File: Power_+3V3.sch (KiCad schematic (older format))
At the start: 10 parts

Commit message: Add files via upload
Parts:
- removed C? (x2): 10u, Capacitor_SMD:C_1206_3216Metric_Pad1.33x1.80mm_HandSolder, symbol Device:C
- removed C?: 0,1, Capacitor_SMD:C_0603_1608Metric_Pad1.08x0.95mm_HandSolder, symbol Device:C
- removed C?: 1u, Capacitor_SMD:C_0603_1608Metric_Pad1.08x0.95mm_HandSolder, symbol Device:C
- removed D?: SMAJ5.0CA, symbol Device:D_TVS
- removed TP?: TestPoint, symbol Connector:TestPoint
- removed U?: AMS1117-3.3, Package_TO_SOT_SMD:SOT-223-3_TabPin2, symbol Regulator_Linear:AMS1117-3.3
- added C? (x2): 10u, Capacitor_SMD:C_1206_3216Metric_Pad1.33x1.80mm_HandSolder, symbol Device:C
- added C?: 0,1, Capacitor_SMD:C_0603_1608Metric_Pad1.08x0.95mm_HandSolder, symbol Device:C
- added C?: 1u, Capacitor_SMD:C_0603_1608Metric_Pad1.08x0.95mm_HandSolder, symbol Device:C
- added TP?: TestPoint, symbol Connector:TestPoint
- added U?: AMS1117-3.3, Package_TO_SOT_SMD:SOT-223-3_TabPin2, symbol Regulator_Linear:AMS1117-3.3
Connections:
- wire segments 18 -> 16

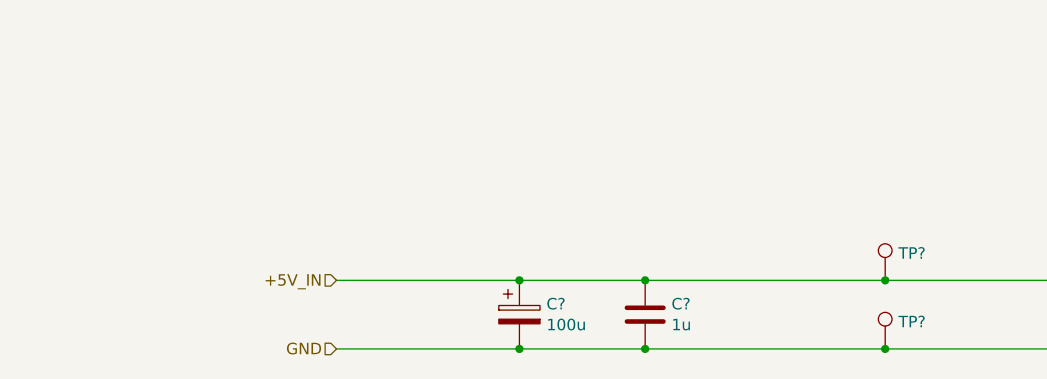
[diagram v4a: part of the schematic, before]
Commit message: Add files via upload
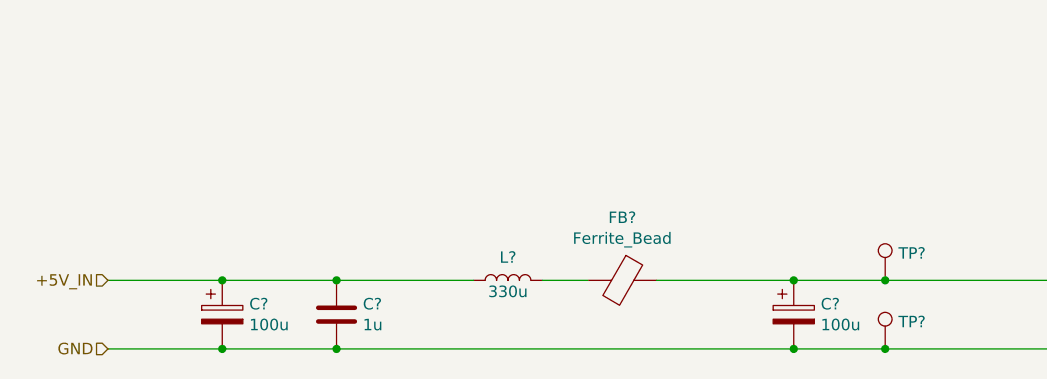
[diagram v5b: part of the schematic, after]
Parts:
- removed C?: 100u, symbol Device:CP
- removed C?: 1u, Capacitor_SMD:C_0603_1608Metric_Pad1.08x0.95mm_HandSolder, symbol Device:C
- added C?: 1u, Capacitor_SMD:C_0603_1608Metric_Pad1.08x0.95mm_HandSolder, symbol Device:C
- added C? (x2): 100u, symbol Device:CP
- added FB?: Ferrite_Bead, symbol Device:Ferrite_Bead
- added L?: 330u, symbol Device:L
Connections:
- net +5V_IN: now also C?.1, C?.1, L?.1; no longer C?.1, TP?.1, U?.3 (VI)
- net GND: now also C?.2, C?.2, C?.2
- new net: C?.1, C?.1, FB?.1, TP?.1, U?.3 (VI)
- new net: FB?.2, L?.2
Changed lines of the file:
@@
 $Descr A4 11693 8268
 encoding utf-8
-Sheet 13 23
+Sheet 11 23
 Title ""
 Date ""
@@
 	1    0    0    -1
 $EndComp
-$Comp
-L Device:C C?
-U 1 1 60E73028
-P 4350 3650
-AR Path="/60E73028" Ref="C?"  Part="1"
-AR Path="/609CA6A8/609D24C0/60E73028" Ref="C?"  Part="1"
-AR Path="/609CA6A8/60A08E0B/60E73028" Ref="C?"  Part="1"
-AR Path="/609CA6A8/60A0A46E/60E73028" Ref="C?"  Part="1"
-AR Path="/609CA6A8/60A0A500/60E73028" Ref="C?"  Part="1"
-AR Path="/609CA6A8/60A0A922/60E73028" Ref="C?"  Part="1"
-AR Path="/609CA6A8/60E73028" Ref="C?"  Part="1"
-AR Path="/609CA6A8/60AE5653/60E73028" Ref="C?"  Part="1"
-AR Path="/609FED99/60E73028" Ref="C?"  Part="1"
-AR Path="/60DF07DE/60E73028" Ref="C?"  Part="1"
-AR Path="/60DF0860/60E73028" Ref="C?"  Part="1"
-AR Path="/60DF1072/60E73028" Ref="C?"  Part="1"
-AR Path="/60DF1160/60E73028" Ref="C?"  Part="1"
-AR Path="/60DF196E/60E73028" Ref="C?"  Part="1"
-AR Path="/60DF212D/60E73028" Ref="C?"  Part="1"
-AR Path="/60E6F2E9/60E73028" Ref="C?"  Part="1"
-F 0 "C?" H 4465 3696 50  0000 L CNN
-F 1 "1u" H 4465 3605 50  0000 L CNN
-F 2 "Capacitor_SMD:C_0603_1608Metric_Pad1.08x0.95mm_HandSolder" H 4388 3500 50  0001 C CNN
-F 3 "~" H 4350 3650 50  0001 C CNN
-	1    4350 3650
-	1    0    0    -1
-$EndComp
-$Comp
-L Device:CP C?
-U 1 1 60DF19BC
-P 3800 3650
-AR Path="/609FED99/60DF19BC" Ref="C?"  Part="1"
-AR Path="/60DF07DE/60DF19BC" Ref="C?"  Part="1"
-AR Path="/60DF0860/60DF19BC" Ref="C?"  Part="1"
-AR Path="/60DF1072/60DF19BC" Ref="C?"  Part="1"
-AR Path="/60DF1160/60DF19BC" Ref="C?"  Part="1"
-AR Path="/60DF196E/60DF19BC" Ref="C?"  Part="1"
-AR Path="/60DF212D/60DF19BC" Ref="C?"  Part="1"
-AR Path="/60E6F2E9/60DF19BC" Ref="C?"  Part="1"
-F 0 "C?" H 3918 3696 50  0000 L CNN
-F 1 "100u" H 3918 3605 50  0000 L CNN
-F 2 "" H 3838 3500 50  0001 C CNN
-F 3 "~" H 3800 3650 50  0001 C CNN
-	1    3800 3650
-	1    0    0    -1
-$EndComp
-Text HLabel 3000 3500 0    50   Input ~ 0
+Text HLabel 2000 3500 0    50   Input ~ 0
 +5V_IN
-Wire Wire Line
-	3000 3500 3800 3500
 Connection ~ 6200 3500
-Connection ~ 3800 3500
-Wire Wire Line
-	3800 3500 4350 3500
-Connection ~ 4350 3500
-Connection ~ 5400 3500
-Wire Wire Line
-	3800 3800 4350 3800
 Connection ~ 6200 3800
-Connection ~ 4350 3800
 Wire Wire Line
 	6800 3800 7400 3800
-Wire Wire Line
-	3000 3800 3800 3800
-Connection ~ 3800 3800
 $Comp
 L Connector:TestPoint TP?
@@
 	1    0    0    -1
 $EndComp
-Connection ~ 5400 3800
 Wire Wire Line
 	7400 3500 7550 3500
@@
 	7550 3500 7800 3500
 Connection ~ 7550 3500
-Text HLabel 3000 3800 0    50   Input ~ 0
+Text HLabel 2000 3800 0    50   Input ~ 0
 GND
 Text Notes 6900 2250 2    197  ~ 0
@@
 	7800 3500 8500 3500
 Connection ~ 7800 3500
-Wire Wire Line
-	4350 3800 5400 3800
-Wire Wire Line
-	4350 3500 5400 3500
+$Comp
+L Device:C C?
+U 1 1 60FB3F89
+P 3000 3650
+AR Path="/60FB3F89" Ref="C?"  Part="1"
+AR Path="/609CA6A8/609D24C0/60FB3F89" Ref="C?"  Part="1"
+AR Path="/609CA6A8/60A08E0B/60FB3F89" Ref="C?"  Part="1"
+AR Path="/609CA6A8/60A0A46E/60FB3F89" Ref="C?"  Part="1"
+AR Path="/609CA6A8/60A0A500/60FB3F89" Ref="C?"  Part="1"
+AR Path="/609CA6A8/60A0A922/60FB3F89" Ref="C?"  Part="1"
+AR Path="/609CA6A8/60FB3F89" Ref="C?"  Part="1"
+AR Path="/609CA6A8/60AE5653/60FB3F89" Ref="C?"  Part="1"
+AR Path="/609FED99/60FB3F89" Ref="C?"  Part="1"
+AR Path="/60DF07DE/60FB3F89" Ref="C?"  Part="1"
+AR Path="/60DF0860/60FB3F89" Ref="C?"  Part="1"
+AR Path="/60DF1072/60FB3F89" Ref="C?"  Part="1"
+AR Path="/60DF1160/60FB3F89" Ref="C?"  Part="1"
+AR Path="/60DF196E/60FB3F89" Ref="C?"  Part="1"
+AR Path="/60DF212D/60FB3F89" Ref="C?"  Part="1"
+AR Path="/60E6F2E9/60FB3F89" Ref="C?"  Part="1"
+AR Path="/60EE89A9/60FB3F89" Ref="C?"  Part="1"
+F 0 "C?" H 3115 3696 50  0000 L CNN
+F 1 "1u" H 3115 3605 50  0000 L CNN
+F 2 "Capacitor_SMD:C_0603_1608Metric_Pad1.08x0.95mm_HandSolder" H 3038 3500 50  0001 C CNN
+F 3 "~" H 3000 3650 50  0001 C CNN
+	1    3000 3650
+	1    0    0    -1
+$EndComp
+$Comp
+L Device:CP C?
+U 1 1 60FB3F8F
+P 2500 3650
+AR Path="/609FED99/60FB3F8F" Ref="C?"  Part="1"
+AR Path="/60DF07DE/60FB3F8F" Ref="C?"  Part="1"
+AR Path="/60DF0860/60FB3F8F" Ref="C?"  Part="1"
+AR Path="/60DF1072/60FB3F8F" Ref="C?"  Part="1"
+AR Path="/60DF1160/60FB3F8F" Ref="C?"  Part="1"
+AR Path="/60DF196E/60FB3F8F" Ref="C?"  Part="1"
+AR Path="/60DF212D/60FB3F8F" Ref="C?"  Part="1"
+AR Path="/60E6F2E9/60FB3F8F" Ref="C?"  Part="1"
+AR Path="/60EE89A9/60FB3F8F" Ref="C?"  Part="1"
+F 0 "C?" H 2618 3696 50  0000 L CNN
+F 1 "100u" H 2618 3605 50  0000 L CNN
+F 2 "" H 2538 3500 50  0001 C CNN
+F 3 "~" H 2500 3650 50  0001 C CNN
+	1    2500 3650
+	1    0    0    -1
+$EndComp
+$Comp
+L Device:CP C?
+U 1 1 60FC0F28
+P 5000 3650
+AR Path="/609FED99/60FC0F28" Ref="C?"  Part="1"
+AR Path="/60DF07DE/60FC0F28" Ref="C?"  Part="1"
+AR Path="/60DF0860/60FC0F28" Ref="C?"  Part="1"
+AR Path="/60DF1072/60FC0F28" Ref="C?"  Part="1"
+AR Path="/60DF1160/60FC0F28" Ref="C?"  Part="1"
+AR Path="/60DF196E/60FC0F28" Ref="C?"  Part="1"
+AR Path="/60DF212D/60FC0F28" Ref="C?"  Part="1"
+AR Path="/60E6F2E9/60FC0F28" Ref="C?"  Part="1"
+AR Path="/60EE89A9/60FC0F28" Ref="C?"  Part="1"
+F 0 "C?" H 5118 3696 50  0000 L CNN
+F 1 "100u" H 5118 3605 50  0000 L CNN
+F 2 "" H 5038 3500 50  0001 C CNN
+F 3 "~" H 5000 3650 50  0001 C CNN
+	1    5000 3650
+	1    0    0    -1
+$EndComp
+$Comp
+L Device:Ferrite_Bead FB?
+U 1 1 60FC2E70
+P 4250 3500
+AR Path="/60DF1072/60FC2E70" Ref="FB?"  Part="1"
+AR Path="/60E6F2E9/60FC2E70" Ref="FB?"  Part="1"
+F 0 "FB?" V 3976 3500 50  0000 C CNN
+F 1 "Ferrite_Bead" V 4067 3500 50  0000 C CNN
+F 2 "" V 4180 3500 50  0001 C CNN
+F 3 "~" H 4250 3500 50  0001 C CNN
+	1    4250 3500
+	0    1    1    0
+$EndComp
+$Comp
+L Device:L L?
+U 1 1 60FC380F
+P 3750 3500
+AR Path="/60DF0860/60FC380F" Ref="L?"  Part="1"
+AR Path="/60DF07DE/60FC380F" Ref="L?"  Part="1"
+AR Path="/60F1863C/60FC380F" Ref="L?"  Part="1"
+F 0 "L?" V 3850 3500 50  0000 C CNN
+F 1 "330u" V 3700 3500 50  0000 C CNN
+F 2 "" H 3750 3500 50  0001 C CNN
+F 3 "~" H 3750 3500 50  0001 C CNN
+	1    3750 3500
+	0    -1   -1   0
+$EndComp
+Wire Wire Line
+	2000 3500 2500 3500
+Connection ~ 2500 3500
+Wire Wire Line
+	2500 3500 3000 3500
+Connection ~ 3000 3500
+Wire Wire Line
+	3000 3500 3600 3500
+Wire Wire Line
+	3900 3500 4100 3500
+Wire Wire Line
+	4400 3500 5000 3500
+Connection ~ 5400 3500
+Connection ~ 5000 3500
+Wire Wire Line
+	5000 3500 5400 3500
+Wire Wire Line
+	2000 3800 2500 3800
+Connection ~ 5400 3800
+Connection ~ 2500 3800
+Wire Wire Line
+	2500 3800 3000 3800
+Connection ~ 3000 3800
+Wire Wire Line
+	3000 3800 5000 3800
+Connection ~ 5000 3800
+Wire Wire Line
+	5000 3800 5400 3800
 $EndSCHEMATC
